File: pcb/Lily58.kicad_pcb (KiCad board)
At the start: 2 copper layers, 142.5 x 106.3 mm, 88 parts, among them J1 LED, J2 4PIN, P1 i2c_pin, P2 i2c_pin, P3 ICSP, SW1 SW_PUSH, SW10 SW_PUSH, SW11 SW_PUSH, SW12 SW_PUSH, SW13 SW_PUSH, SW14 SW_PUSH, SW15 SW_PUSH, SW16 SW_PUSH, SW17 SW_PUSH, SW18 SW_PUSH, SW19 SW_PUSH, SW2 SW_PUSH, SW20 SW_PUSH, SW21 SW_PUSH, SW22 SW_PUSH, SW23 SW_PUSH, SW24 SW_PUSH, SW25 SW_PUSH, SW26 SW_PUSH, SW27 SW_PUSH, SW28 SW_PUSH, SW29 SW_PUSH, SW3 SW_PUSH, SW4 SW_PUSH, SW5 SW_PUSH, SW6 SW_PUSH, SW7 SW_PUSH, SW8 SW_PUSH, SW9 SW_PUSH, U1 ProMicro

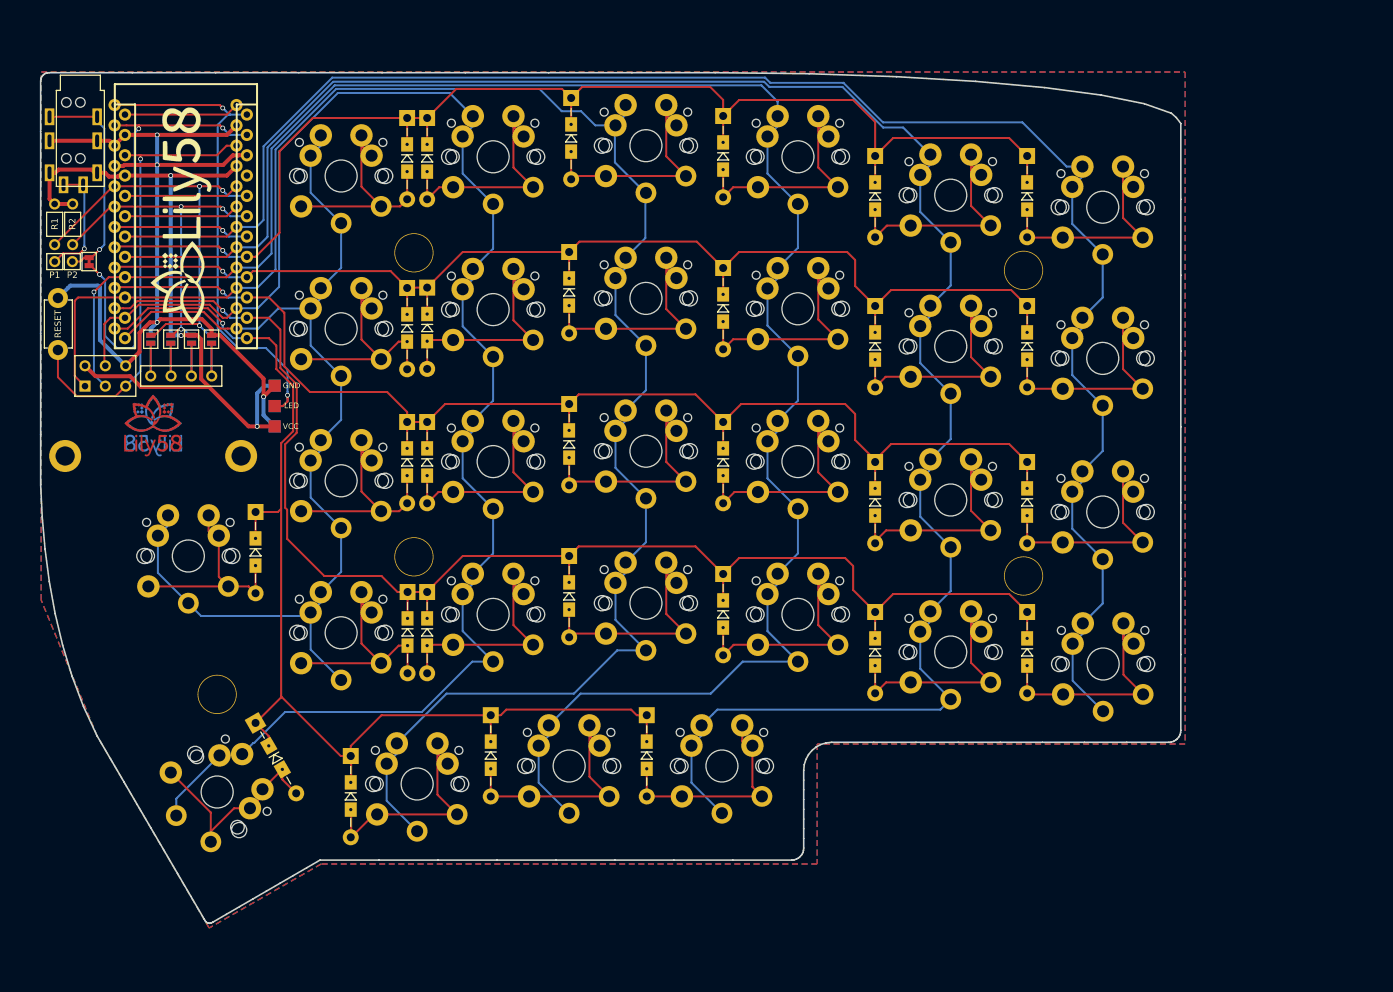
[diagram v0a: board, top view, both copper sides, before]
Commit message: update
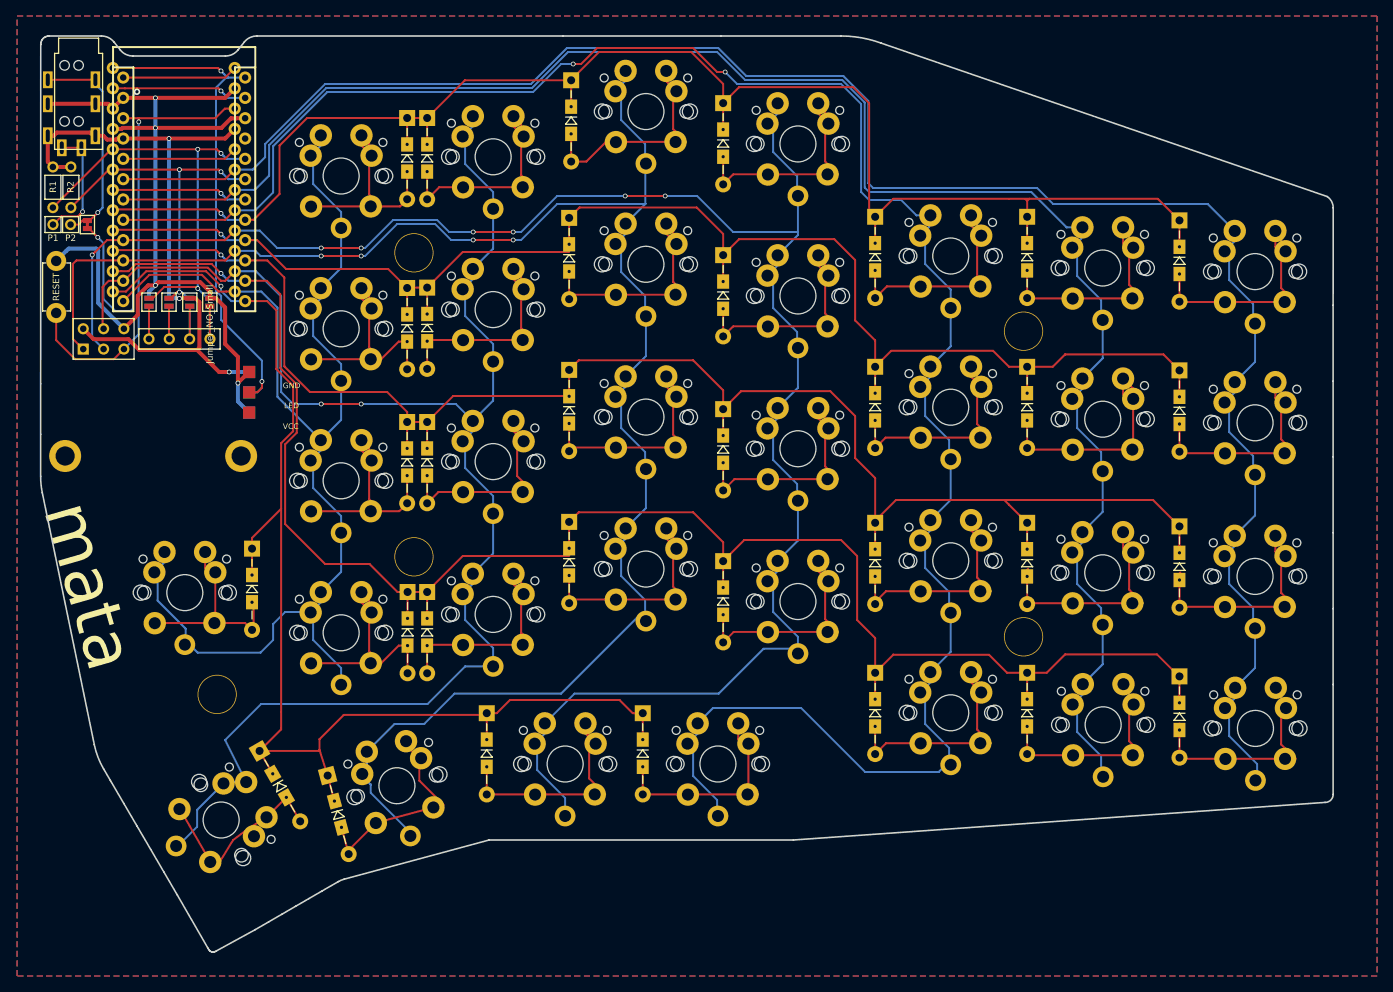
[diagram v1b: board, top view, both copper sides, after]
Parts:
- removed G*** (x2): LOGO, Lily58-footprint:lily58_logo_2
- removed G*** (x2): LOGO, Lily58-footprint:lily58_logo_3
- added D12: D, Lily58-footprint:Diode_TH_SOD123, F.Cu at (225.3, 79.3)
- added D18: D, Lily58-footprint:Diode_TH_SOD123, F.Cu at (225.3, 98.8)
- added D24: D, Lily58-footprint:Diode_TH_SOD123, F.Cu at (225.3, 117.6)
- added D6: D, Lily58-footprint:Diode_TH_SOD123, F.Cu at (225.3, 60.6)
- added SW12: SW_PUSH, Lily58-footprint:MX_PG1350-Under_FLIP_HOLES_18mm, F.Cu at (234.7, 80.9)
- added SW18: SW_PUSH, Lily58-footprint:MX_PG1350-Under_FLIP_HOLES_18mm, F.Cu at (234.7, 100.1)
- added SW24: SW_PUSH, Lily58-footprint:MX_PG1350-Under_FLIP_HOLES_18mm, F.Cu at (234.8, 119.1)
- added SW6: SW_PUSH, Lily58-footprint:MX_PG1350-Under_FLIP_HOLES_18mm, F.Cu at (234.7, 62.0)
- JP1, JP2, JP3, JP4, JP5, JP6, JP7, JP8: value (none) -> Jumper_NO_Small
- moved SW11 7.60 mm to (196.7, 78.9)
- moved SW12 7.60 mm to (215.7, 80.4)
- moved TH4 7.60 mm to (205.8, 69.4)
- moved D5 7.60 mm to (187.2, 60.1)
- moved D6 7.60 mm to (206.2, 60.1)
- moved SW5 7.60 mm to (196.7, 60.0)
- moved SW6 7.60 mm to (215.7, 61.5)
- moved D11 7.60 mm to (187.2, 78.8)
- moved D12 7.60 mm to (206.2, 78.8)
- moved D17 7.60 mm to (187.2, 98.3)
- moved D18 7.60 mm to (206.2, 98.3)
- moved D23 7.60 mm to (187.2, 117.1)
- moved D24 7.60 mm to (206.2, 117.1)
- moved SW17 7.60 mm to (196.7, 98.1)
- moved SW18 7.60 mm to (215.7, 99.6)
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- renumbered OLED to P4
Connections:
- JP1 pad 1: Net-(JP1-Pad1) -> (no net)
- JP2 pad 1: Net-(JP2-Pad1) -> (no net)
- JP3 pad 1: Net-(JP3-Pad1) -> (no net)
- JP4 pad 1: Net-(JP4-Pad1) -> (no net)
- JP5 pad 1: Net-(JP1-Pad1) -> Net-(P4-P4)
- JP6 pad 1: Net-(JP2-Pad1) -> Net-(P4-P3)
- JP7 pad 1: Net-(JP3-Pad1) -> Net-(P4-P2)
- JP8 pad 1: Net-(JP4-Pad1) -> Net-(P4-P1)
- P3 pad 1: col3 -> col4
- P3 pad 3: col2 -> col3
- P3 pad 4: col4 -> col5
- P4 pad 1: Net-(JP4-Pad1) -> Net-(P4-P1)
- P4 pad 2: Net-(JP3-Pad1) -> Net-(P4-P2)
- P4 pad 3: Net-(JP2-Pad1) -> Net-(P4-P3)
- P4 pad 4: Net-(JP1-Pad1) -> Net-(P4-P4)
- SW1 pad 1: col5 -> col6
- SW10 pad 1: col2 -> col3
- SW11 pad 1: col1 -> col2
- SW12 pad 1: col0 -> col1
- SW13 pad 1: col5 -> col6
- SW14 pad 1: col4 -> col5
- SW15 pad 1: col3 -> col4
- SW16 pad 1: col2 -> col3
- SW17 pad 1: col1 -> col2
- SW18 pad 1: col0 -> col1
- SW19 pad 1: col5 -> col6
- SW2 pad 1: col4 -> col5
- SW20 pad 1: col4 -> col5
- SW21 pad 1: col3 -> col4
- SW22 pad 1: col2 -> col3
- SW23 pad 1: col1 -> col2
- SW24 pad 1: col0 -> col1
- SW25 pad 1: col5 -> col6
- SW26 pad 1: col4 -> col5
- SW27 pad 1: col3 -> col4
- SW28 pad 1: col2 -> col3
- SW29 pad 1: col1 -> col2
- SW3 pad 1: col3 -> col4
- SW4 pad 1: col2 -> col3
- SW5 pad 1: col1 -> col2
- SW6 pad 1: col0 -> col1
- SW7 pad 1: col5 -> col6
- SW8 pad 1: col4 -> col5
- SW9 pad 1: col3 -> col4
- U1 pad 13: col5 -> col6
- U1 pad 14: col4 -> col5
- U1 pad 15: col3 -> col4
- U1 pad 16: col2 -> col3
- U1 pad 17: col1 -> col2
- U1 pad 18: col0 -> col1
- U1 pad 19: Net-(U1-Pad19) -> col0
- U1 pad 20: Net-(U1-Pad20) -> unconnected-(U1-A3(PF4)-Pad20)
- U1 pad 24: Net-(U1-Pad24) -> unconnected-(U1-RAW-Pad24)_0
- U1 pad 7: Net-(U1-Pad7) -> unconnected-(U1-D4(PD4)-Pad7)_0
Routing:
- net col6: track 0.00 -> 154.7 mm
- net col5: track 135.9 -> 206.0 mm, vias 0 -> 2
- net (no net): track 0.00 -> 45.9 mm, vias 0 -> 1
- net row2: track 155.9 -> 199.0 mm
- net row3: track 176.5 -> 217.0 mm
- net row1: track 146.6 -> 182.8 mm
- net row0: track 160.9 -> 193.5 mm
- net Net-(D14-A): track 0.00 -> 31.4 mm
- net Net-(D7-A): track 0.00 -> 31.3 mm
- net Net-(D21-A): track 0.00 -> 30.6 mm
- net Net-(D28-A): track 0.00 -> 27.9 mm
- net col0: track 217.9 -> 241.2 mm
- net col1: track 245.7 -> 223.9 mm
- net col4: track 204.8 -> 222.4 mm, vias 0 -> 4
- net Net-(U1-Pad7): track 17.0 -> 0.00 mm, vias 1 -> 0
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- added copper zone on B.Cu, net (none)
- added copper zone on F.Cu, net (none)
- removed copper zone on B.Cu, net GND
- removed copper zone on F.Cu, net GND
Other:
- board size 142.5 x 106.3 mm -> 161.6 x 114.5 mm
- net class Default removed
- net class GND removed
- net class VCC removed
- board text added: "0.2000 mm / 0.0000 mm"
- board text added: "0.3000 mm"
- board text added: "1.6000 mm"
- board text added: "161.5706 mm x 114.5072 mm"
- board text added: "2"
- board text added: "BOARD CHARACTERISTICS"
- board text added: "Board Thickness:"
- board text added: "Board overall dimensions:"
- board text added: "Castellated pads:"
- board text added: "Copper Finish:"
- board text added: "Copper Layer Count:"
- board text added: "Edge card connectors:"
- board text added: "Impedance Control:"
- board text added: "Min hole diameter:"
- board text added: "Min track/spacing:"
- board text added: "Neko"
- board text added: "No"
- board text added: "None"
- board text added: "Plated Board Edge:"
- board text added: "mata"
